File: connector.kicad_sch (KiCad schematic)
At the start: 2 parts, among them J401 AXK500137YG, J402 AXK500137YG

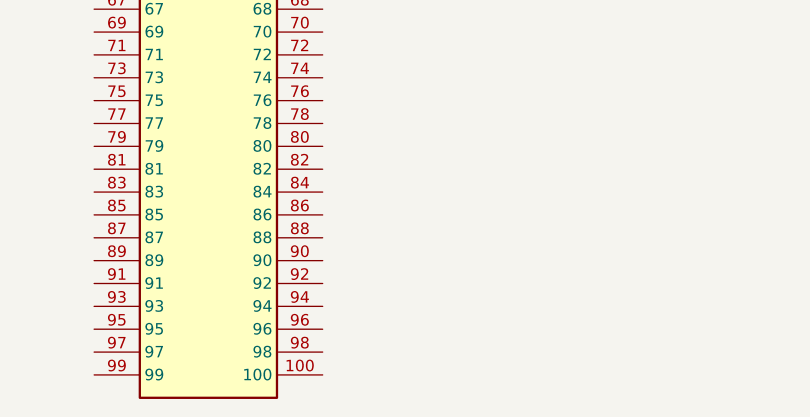
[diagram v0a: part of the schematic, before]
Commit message: feat: need finish power layout
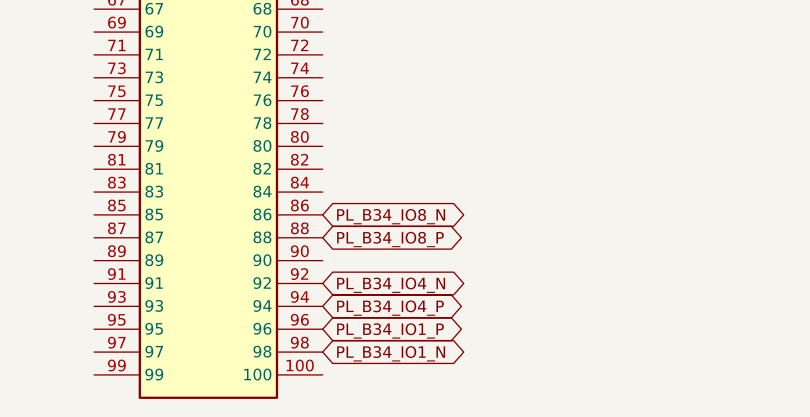
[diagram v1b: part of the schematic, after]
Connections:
- net PL_B34_IO8_N: now reaches J401.86
- net PL_B34_IO8_P: now reaches J401.88
- net PL_B34_IO4_N: now reaches J401.92
- net PL_B34_IO4_P: now reaches J401.94
- net PL_B34_IO1_P: now reaches J401.96
- net PL_B34_IO1_N: now reaches J401.98
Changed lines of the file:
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@@
+		)
+	)
+	(global_label "PL_B34_IO4_N"
+		(shape bidirectional)
+		(at 90.17 160.02 0)
+		(effects
+			(font
+				(size 1.27 1.27)
+			)
+			(justify left)
+		)
+		(property "Intersheetrefs" "${INTERSHEET_REFS}"
+			(at 90.17 160.02 0)
+			(hide yes)
+			(show_name no)
+			(do_not_autoplace no)
+			(effects
+				(font
+					(size 1.27 1.27)
+				)
+			)
+		)
+	)
+	(global_label "PL_B34_IO1_P"
+		(shape bidirectional)
+		(at 90.17 165.1 0)
+		(effects
+			(font
+				(size 1.27 1.27)
+			)
+			(justify left)
+		)
+		(property "Intersheetrefs" "${INTERSHEET_REFS}"
+			(at 90.17 165.1 0)
+			(hide yes)
+			(show_name no)
+			(do_not_autoplace no)
+			(effects
+				(font
+					(size 1.27 1.27)
+				)
+			)
+		)
+	)
+	(global_label "PL_B34_IO1_N"
+		(shape bidirectional)
+		(at 90.17 167.64 0)
+		(effects
+			(font
+				(size 1.27 1.27)
+			)
+			(justify left)
+		)
+		(property "Intersheetrefs" "${INTERSHEET_REFS}"
+			(at 90.17 167.64 0)
+			(hide yes)
+			(show_name no)
+			(do_not_autoplace no)
+			(effects
+				(font
+					(size 1.27 1.27)
+				)
+			)
+		)
+	)
+	(global_label "PL_B34_IO4_P"
+		(shape bidirectional)
+		(at 90.17 162.56 0)
+		(effects
+			(font
+				(size 1.27 1.27)
+			)
+			(justify left)
+		)
+		(property "Intersheetrefs" "${INTERSHEET_REFS}"
+			(at 90.17 162.56 0)
+			(hide yes)
+			(show_name no)
+			(do_not_autoplace no)
+			(effects
+				(font
+					(size 1.27 1.27)
+				)
+			)
+		)
+	)
+	(global_label "PL_B34_IO8_P"
+		(shape bidirectional)
+		(at 90.17 154.94 0)
+		(effects
+			(font
+				(size 1.27 1.27)
+			)
+			(justify left)
+		)
+		(property "Intersheetrefs" "${INTERSHEET_REFS}"
+			(at 90.17 154.94 0)
+			(hide yes)
+			(show_name no)
+			(do_not_autoplace no)
+			(effects
+				(font
+					(size 1.27 1.27)
+				)
+			)
+		)
+	)
+	(global_label "PL_B34_IO8_N"
+		(shape bidirectional)
+		(at 90.17 152.4 0)
+		(effects
+			(font
+				(size 1.27 1.27)
+			)
+			(justify left)
+		)
+		(property "Intersheetrefs" "${INTERSHEET_REFS}"
+			(at 90.17 152.4 0)
+			(hide yes)
+			(show_name no)
+			(do_not_autoplace no)
+			(effects
+				(font
+					(size 1.27 1.27)
+				)
+			)
 		)
 	)
